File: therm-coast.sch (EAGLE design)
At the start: 20 parts, among them U1 ATTINY85-20SU

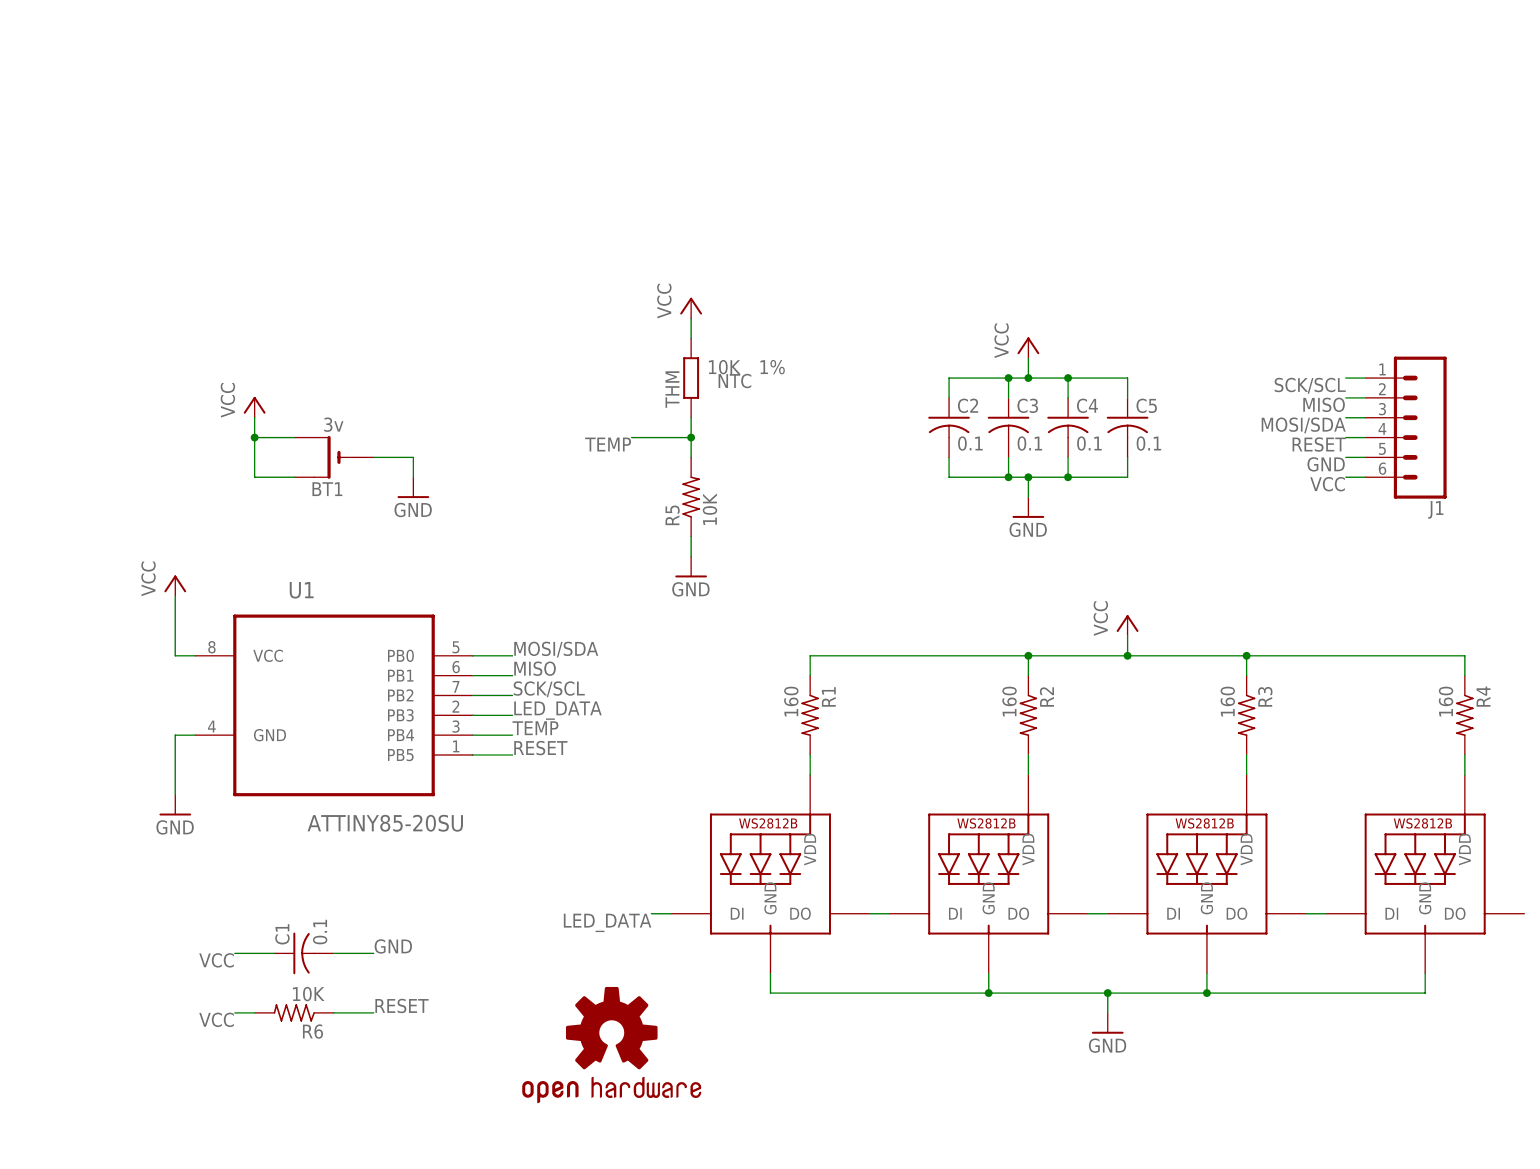
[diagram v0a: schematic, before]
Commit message: Cleaned up for entry
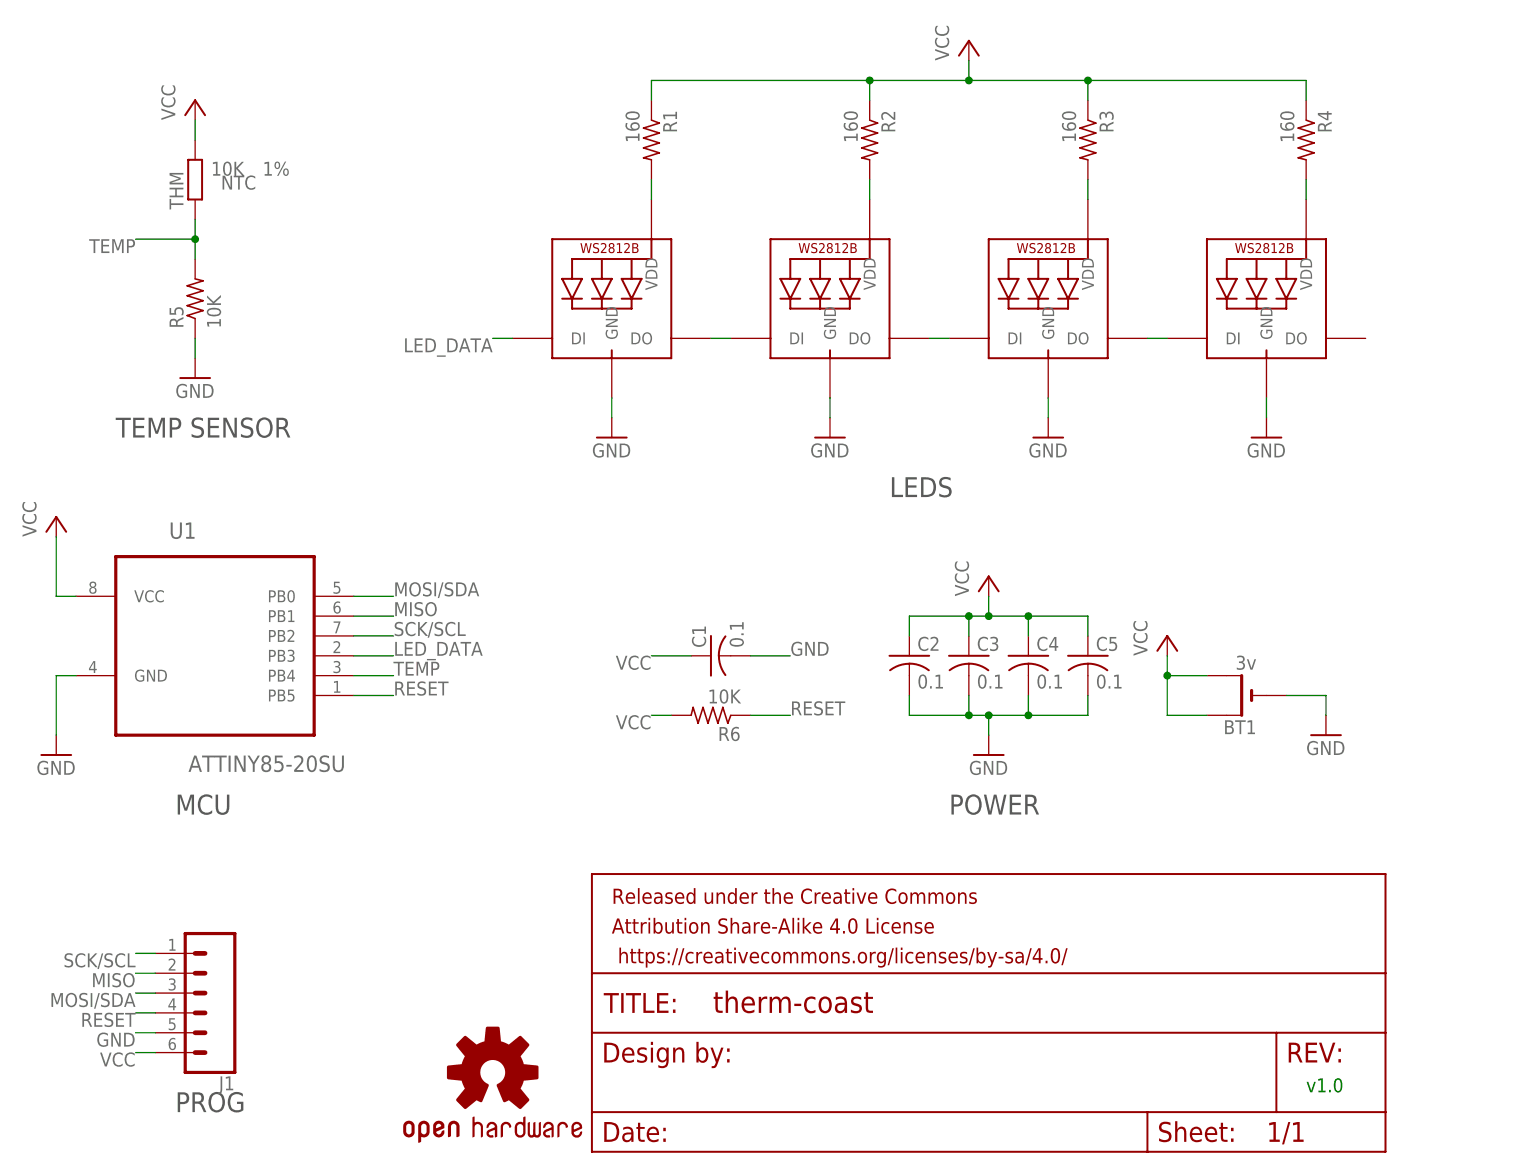
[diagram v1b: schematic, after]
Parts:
- added FRAME1: FRAME-LETTER, SparkFun-Aesthetics:FRAME-LETTER
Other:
- note added: "LEDS"
- note added: "MCU"
- note added: "POWER"
- note added: "PROG"
- note added: "Ray Olsen @_rayolsen https://github.com/rayolsen/Therm-Coaster"
- note added: "TEMP SENSOR"
- note added: "v1.0"
- moved on the sheet: BT1, C1, C2, C3, C4, C5, J1, R1, R2, R3, R4, R5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
